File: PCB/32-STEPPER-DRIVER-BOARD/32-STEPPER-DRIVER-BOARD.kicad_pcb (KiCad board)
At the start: 2 copper layers, 100 x 100 mm, 412 parts, among them J1 MEC2-30-01-X-TH1-NP-WT, J2 MEC2-30-01-X-TH1-NP-WT, J3 MEC2-30-01-X-TH1-NP-WT, J4 MEC2-30-01-X-TH1-NP-WT, U1 74HC595, U10 74HC595, U11 74HC595, U12 74HC595, U13 74HC595, U14 74HC595, U15 74HC595, U16 74HC595, U17 74HC595, U18 74HC595, U19 74HC595, U2 74HC595, U20 74HC595, U21 74HC595, U22 74HC595, U23 74HC595, U24 74HC595, U3 74HC595, U4 74HC595, U5 74HC595, U6 74HC595, U7 74HC595, U8 74HC595, U9 74HC595

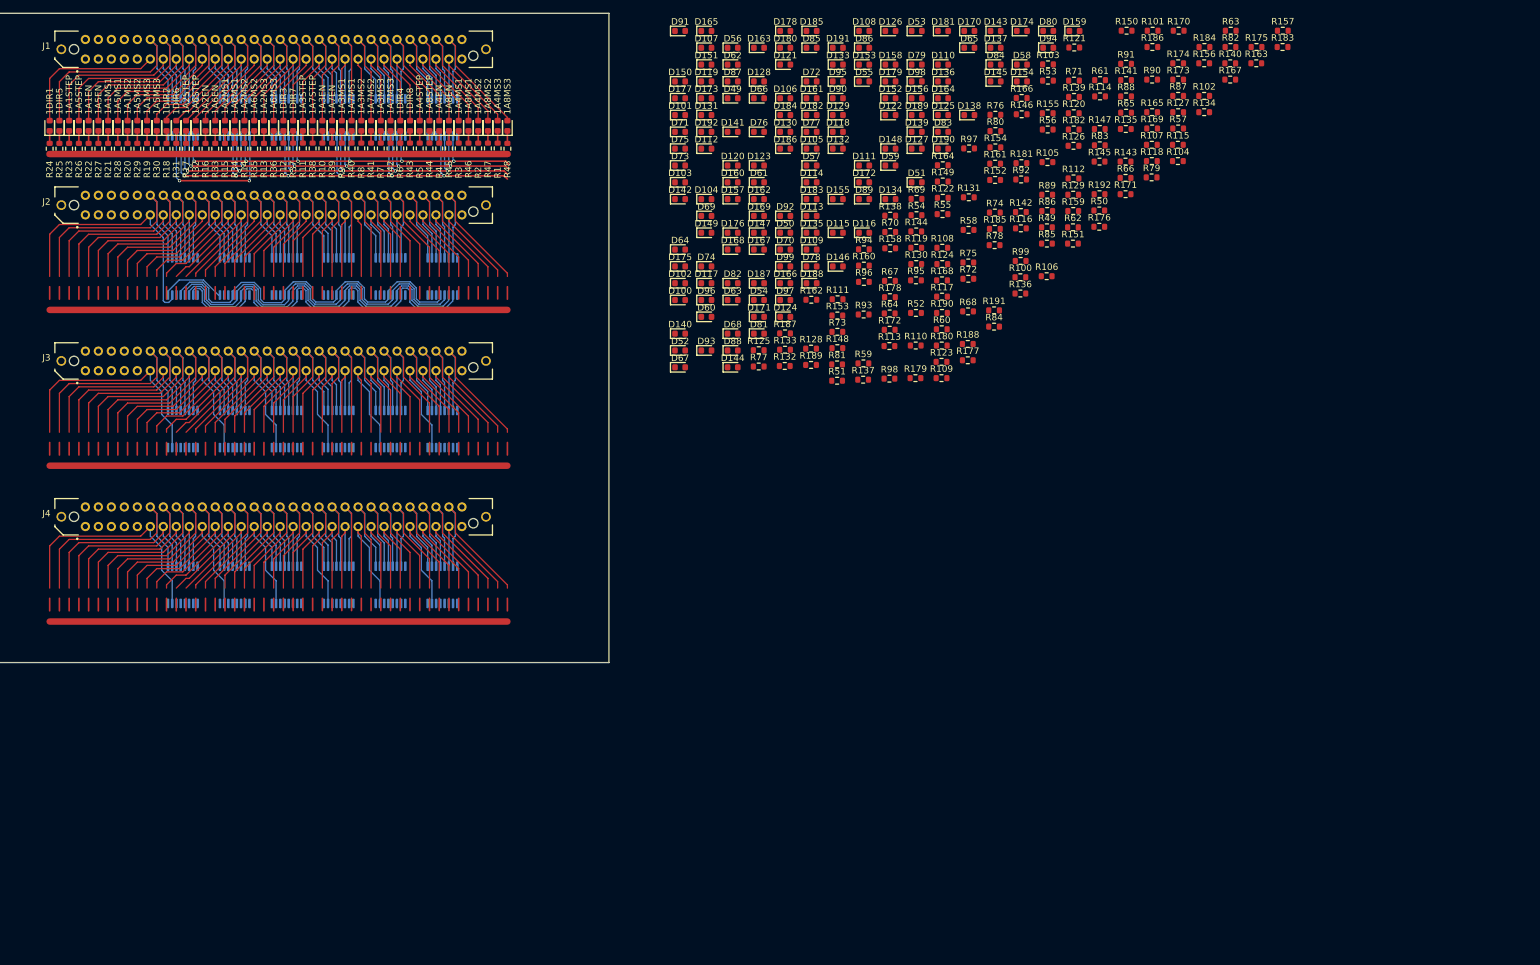
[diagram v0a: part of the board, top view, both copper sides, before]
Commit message: progress
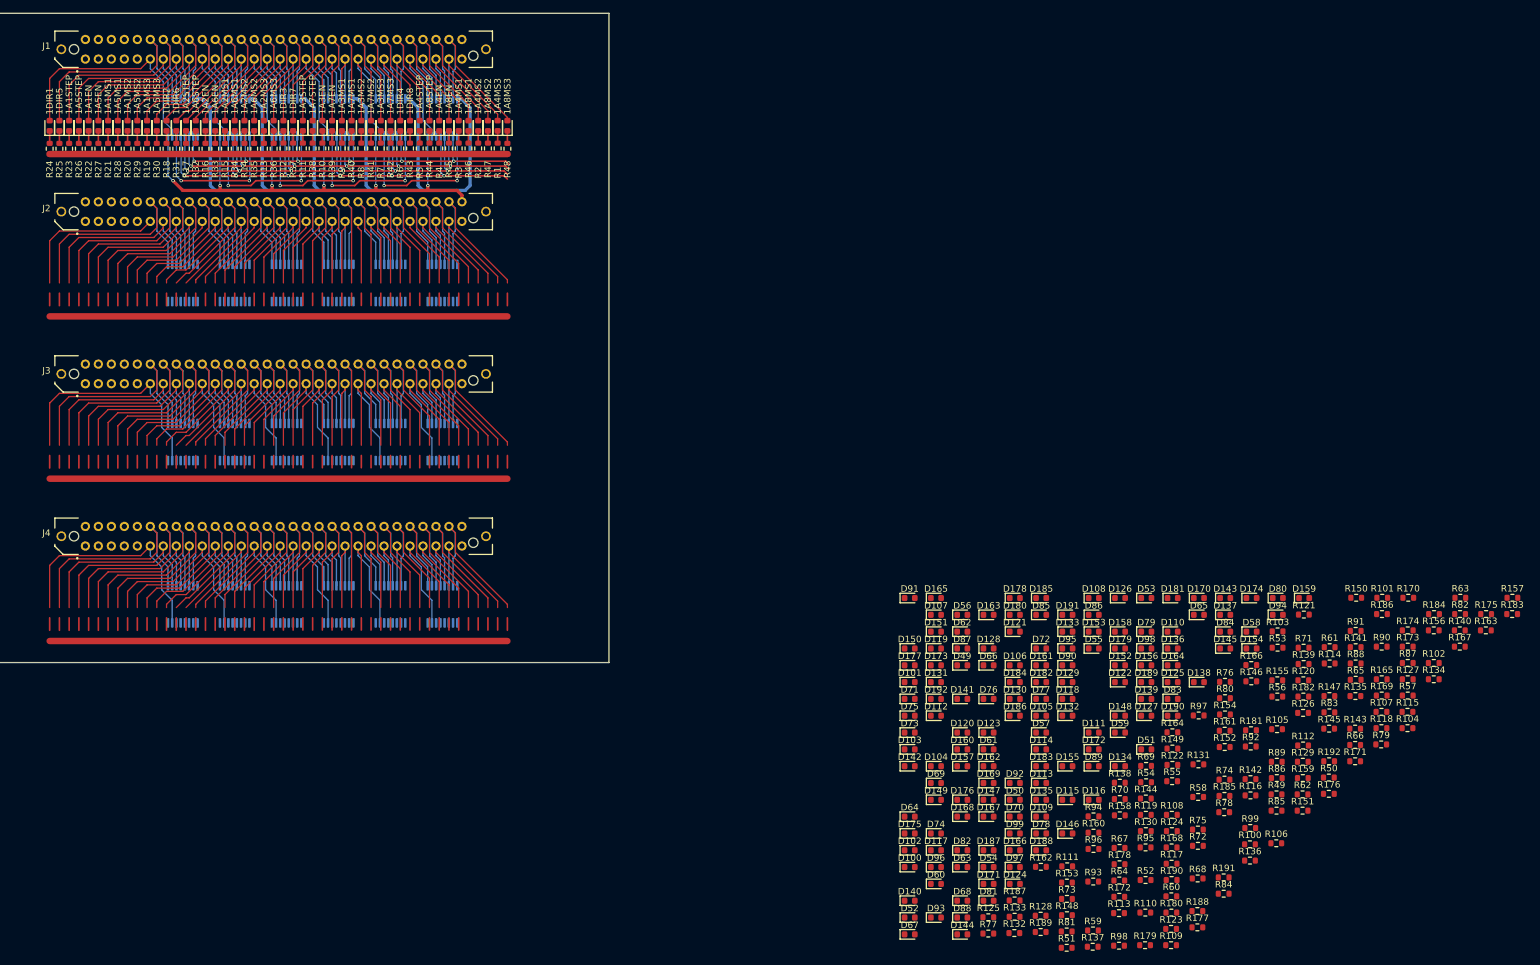
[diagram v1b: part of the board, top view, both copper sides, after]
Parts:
- moved D100 94.2 mm to (187.0, 145.5)
- moved D101 94.2 mm to (187.0, 117.0)
- moved D102 94.2 mm to (187.0, 142.9)
- moved D103 94.2 mm to (187.0, 127.3)
- moved D105 94.2 mm to (207.2, 122.2)
- moved D108 94.2 mm to (215.3, 104.0)
- moved D111 94.2 mm to (215.3, 124.8)
- moved D113 94.2 mm to (207.2, 132.5)
- moved D114 94.2 mm to (207.2, 127.3)
- moved D116 94.2 mm to (215.3, 135.1)
- moved D120 94.2 mm to (195.1, 124.8)
- moved D122 94.2 mm to (219.4, 117.0)
- moved D123 94.2 mm to (199.1, 124.8)
- moved D125 94.2 mm to (227.5, 117.0)
- moved D126 94.2 mm to (219.4, 104.0)
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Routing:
- net GND: track 282.0 -> 414.1 mm
- net +5V: track 10.3 -> 95.6 mm, vias 0 -> 6
- net ~{SRCLR}: track 135.4 -> 72.3 mm
- net SRCLK: track 137.6 -> 77.7 mm
- net RCLK: track 142.4 -> 82.8 mm
- net ~{OE}: track 144.4 -> 88.2 mm
- net Net-(U4-Pad9): track 0.00 -> 26.1 mm, vias 0 -> 2
- net Net-(U4-Pad14): track 0.00 -> 26.1 mm, vias 0 -> 2
- net Net-(U3-Pad14): track 0.00 -> 26.1 mm, vias 0 -> 2
- net Net-(U2-Pad14): track 0.00 -> 26.1 mm, vias 0 -> 2
- net 2DIR1: track 39.6 -> 23.2 mm
- net 1DIR3: track 10.9 -> 24.2 mm
- net 1A4EN: track 11.3 -> 24.6 mm
- net 1A2EN: track 12.6 -> 25.8 mm
- net 1A1MS2: track 17.5 -> 30.7 mm
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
